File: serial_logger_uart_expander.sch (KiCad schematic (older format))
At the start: 60 parts, among them J1 CN6, J2 CN8, J3 CN5, J4 CN9, J5 Screw_Terminal_01x10, J6 Screw_Terminal_01x10, U1 M74HC4851, U10 2N7002PS, U11 2N7002PS, U12 2N7002PS, U13 2N7002PS, U14 ESDA17-5SC6, U15 NRF24L01_Breakout, U2 M74HC4851, U3 ESDA17-5SC6, U4 ESDA17-5SC6, U5 ESDA17-5SC6

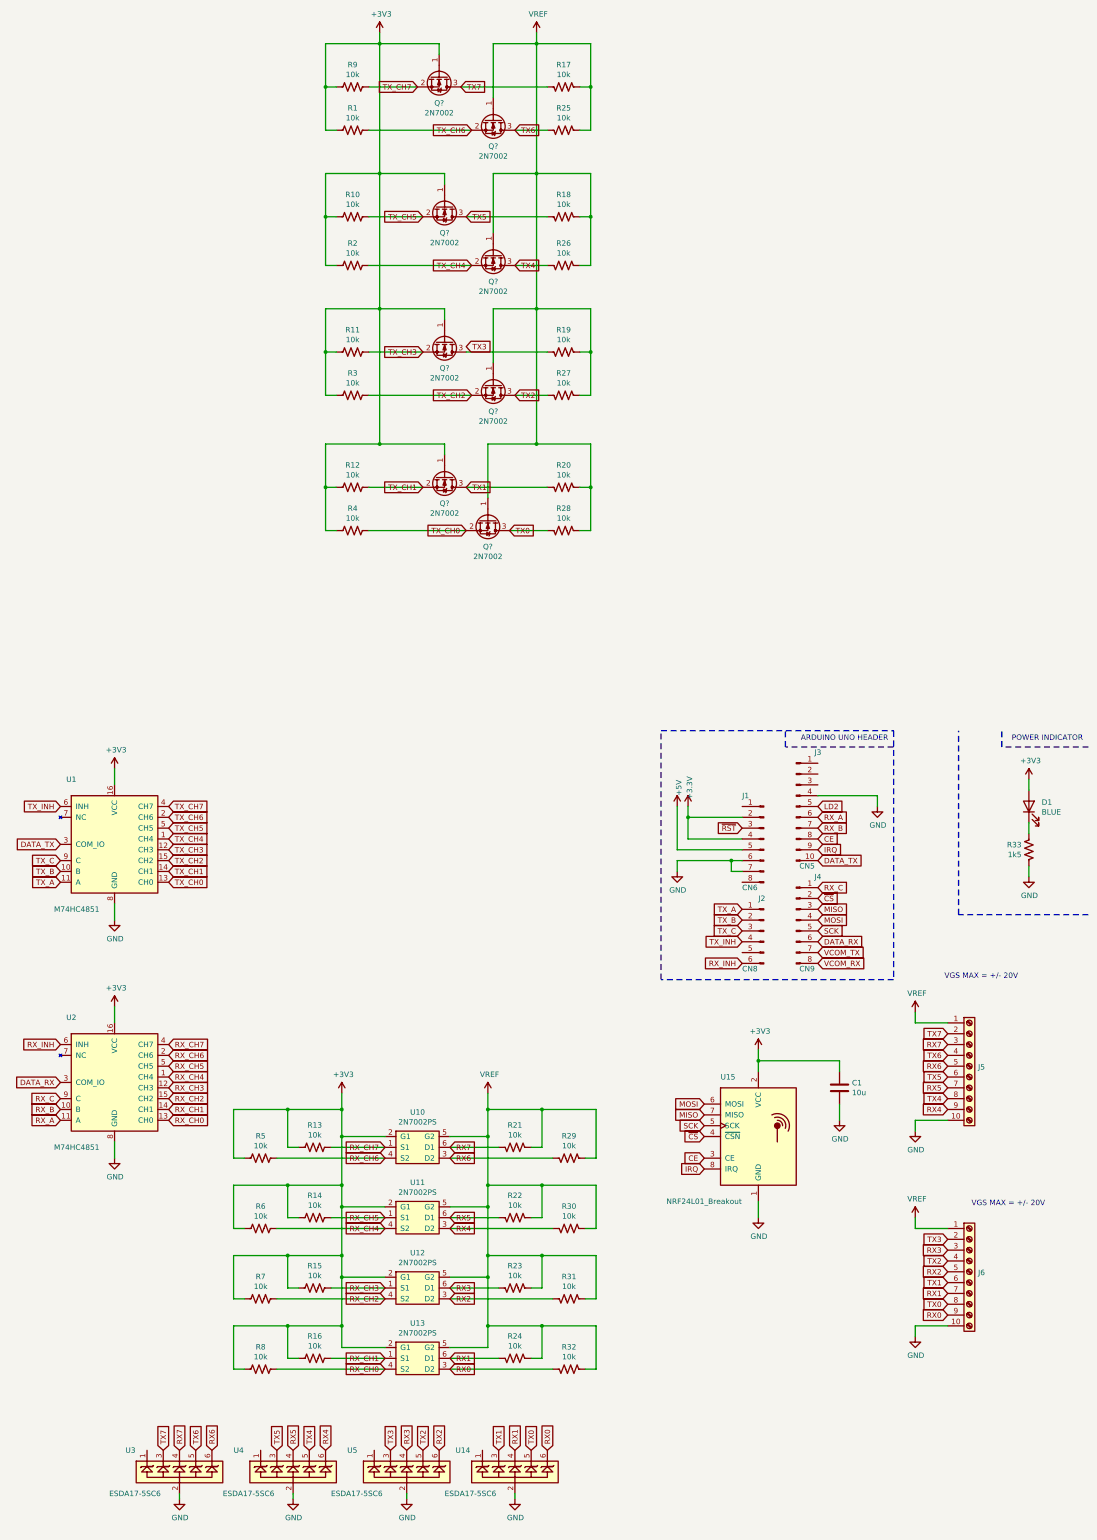
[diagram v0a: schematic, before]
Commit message: completed v0.1 design with 2n7002; no BOM or gerbers
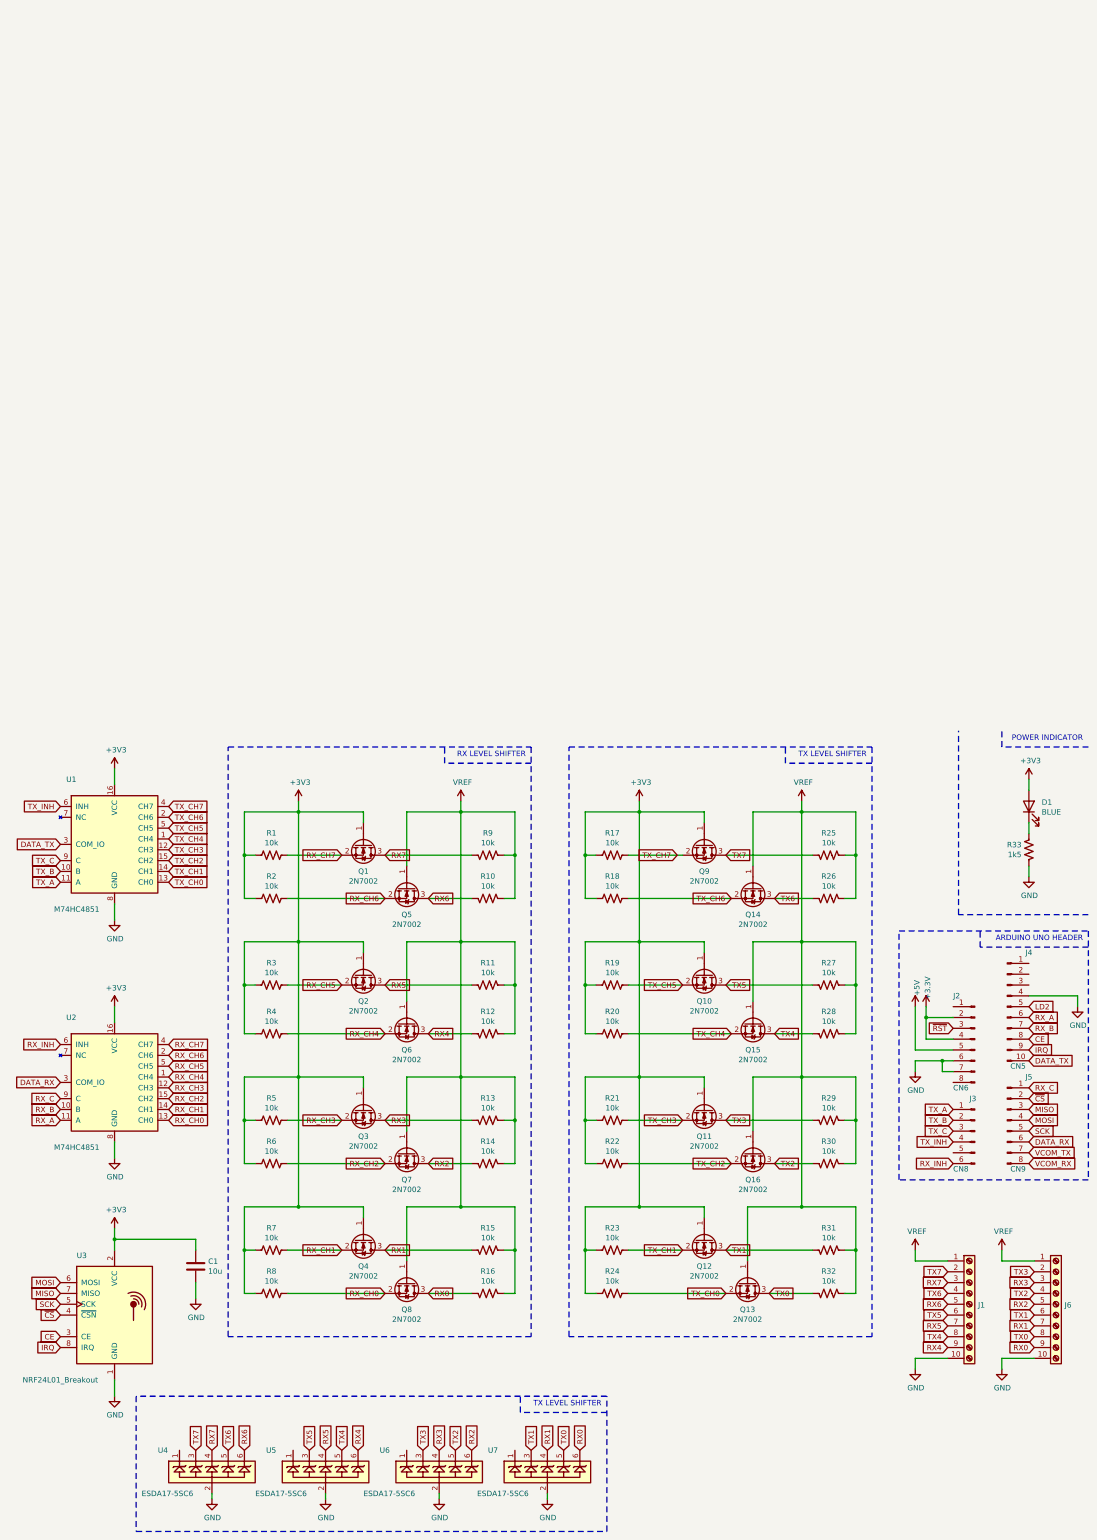
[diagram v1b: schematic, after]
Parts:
- removed U10, U11, U12, U13: 2N7002PS, my_lib:2N7002PS_NEXPERA_SOT-363, symbol my_lib:2N7002PS
- added Q1, Q2, Q3, Q4, Q5, Q6, Q7, Q8: 2N7002, Package_TO_SOT_SMD:SOT-23, symbol Transistor_FET:2N7002
- gave numbers to parts that had none: 8
- renumbered J5 to J1, J1 to J2, J2 to J3, J3 to J4, J4 to J5, R13 to R1, R29 to R10, R22 to R11, R30 to R12, R23 to R13, R31 to R14, R24 to R15, R32 to R16, R9 to R17, R1 to R18, R10 to R19, R5 to R2, R2 to R20, R11 to R21, R3 to R22, R12 to R23, R4 to R24, R17 to R25, R25 to R26, R18 to R27, R26 to R28, R19 to R29, R14 to R3, R27 to R30, R20 to R31, R28 to R32, R6 to R4, R15 to R5, R7 to R6, R16 to R7, R21 to R9, U15 to U3, U3 to U4, U4 to U5, U5 to U6, U14 to U7
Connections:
- net +3V3: now also Q1.1 (G), Q2.1 (G), Q3.1 (G), Q4.1 (G)
- net RX0: now also Q8.3 (D)
- net RX1: now also Q4.3 (D)
- net RX2: now also Q7.3 (D)
- net RX3: now also Q3.3 (D)
- net RX4: now also Q6.3 (D)
- net RX5: now also Q2.3 (D)
- net RX6: now also Q5.3 (D)
- net RX7: now also Q1.3 (D)
- net RX_CH0: now also Q8.2 (S)
- net RX_CH1: now also Q4.2 (S)
- net RX_CH2: now also Q7.2 (S)
- net RX_CH3: now also Q3.2 (S)
- net RX_CH4: now also Q6.2 (S)
- net RX_CH5: now also Q2.2 (S)
- net RX_CH6: now also Q5.2 (S)
- net RX_CH7: now also Q1.2 (S)
- net TX3: now also Q11.3 (D), R29.2
- net VBUS: now also Q5.1 (G), Q6.1 (G), Q7.1 (G), Q8.1 (G)
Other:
- note added: "RX LEVEL SHIFTER"
- note added: "TX LEVEL SHIFTER"
- note removed: "VGS MAX = +/- 20V"
- moved on the sheet: C1, J1, J2, J3, J4, J5, J6, Q10, Q11, Q12, Q13, Q14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
